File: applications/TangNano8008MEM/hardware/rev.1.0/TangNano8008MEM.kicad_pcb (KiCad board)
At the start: 2 copper layers, 99.1 x 99.1 mm, 43 parts, among them J1 Barrel_Jack_Switch, J2 VCC_FPGA, J3 CPU Vcc, J4 TangNano20K5VInterface, J5 Conn_01x20, J6 Conn_01x20, J7 UART, J8 Conn_01x30, J9 Conn_01x30, SW1 SW_SPDT, SW2 INIT, SW3 HALT, U1 DCJ11, Y1 18MHz

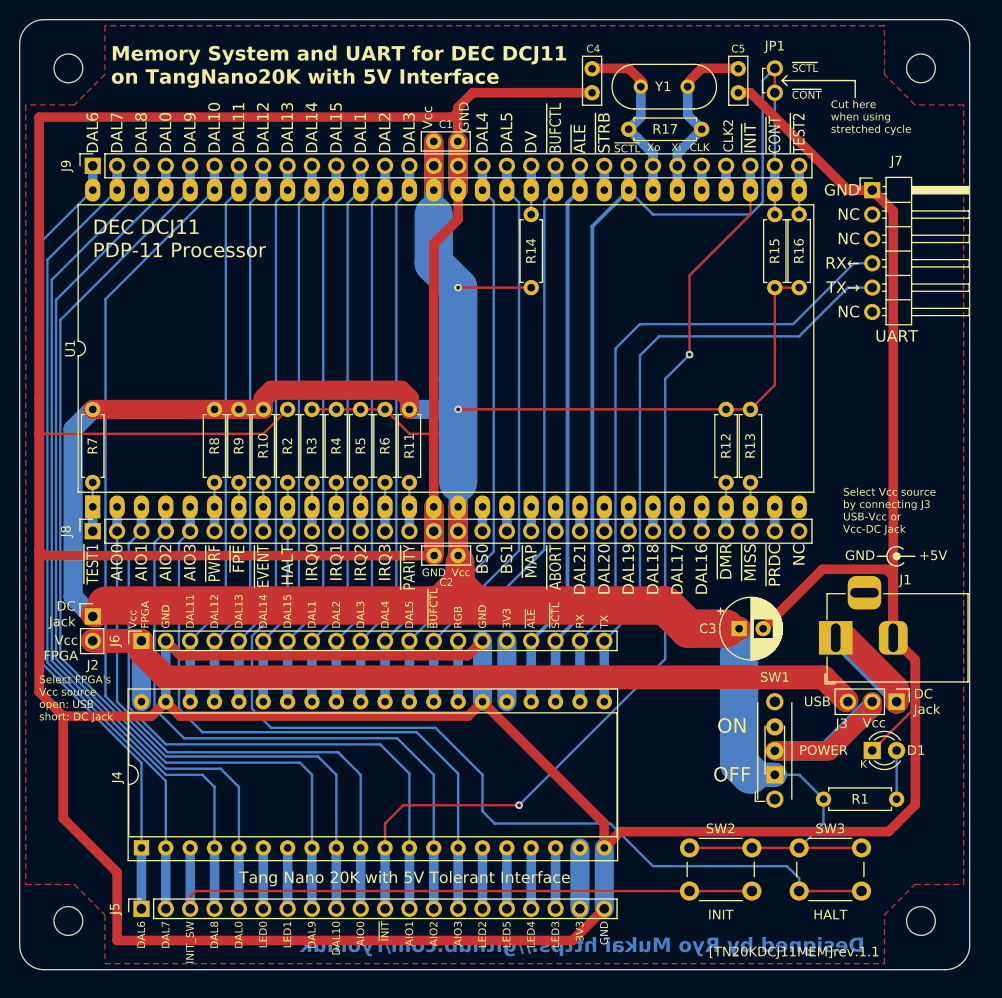
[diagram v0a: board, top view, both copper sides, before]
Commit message: PCB for 8008 updated
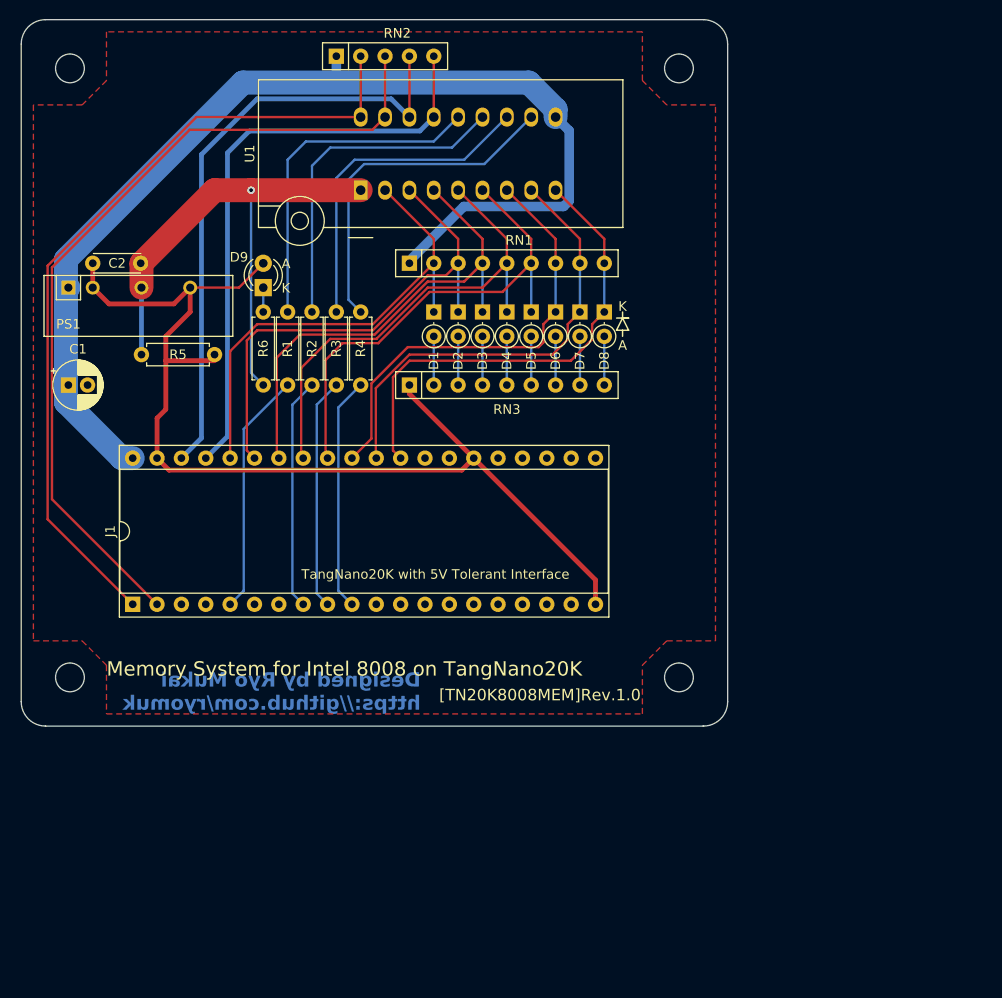
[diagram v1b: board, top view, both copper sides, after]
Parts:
- removed C3: 47uF, 000_MyFootprint:CP_Radial_D6.3mm_P2.50mm
- removed C4, C5: 68p, 000_MyFootprint:C_Disc_D5.0mm_W2.5mm_P2.50mm
- removed J2: VCC_FPGA, 000_MyFootprint:PinHeader_1x02_P2.54mm_Vertical
- removed J3: CPU Vcc, 000_MyFootprint:PinHeader_1x03_P2.54mm_Vertical
- removed J4: TangNano20K5VInterface, 000_MyFootprint:DIP-40_W15.24mm_Socket
- removed J5, J6: Conn_01x20, 000_MyFootprint:PinSocket_1x20_P2.54mm_Vertical
- removed J7: UART, 000_MyFootprint:PinHeader_1x06_P2.54mm_Horizontal
- removed J8, J9: Conn_01x30, 000_MyFootprint:PinSocket_1x30_P2.54mm_Vertical
- removed JP1: SCTL_CONT, 000_MyFootprint:JumperedPinHeader_1x02_P2.54mm_Vertical
- removed R10, R11, R12, R13, R14, R15, R16, R7, R8, R9: 100k, 000_MyFootprint:R_Axial_DIN0207_L6.3mm_D2.5mm_P7.62mm_Horizontal
- removed R17: 1M, 000_MyFootprint:R_Axial_DIN0207_L6.3mm_D2.5mm_P7.62mm_Horizontal
- removed the REF** at (94.0, 94.0)
- removed the REF** at (5.08, 5.08)
- removed the REF** at (91.4, 55.9)
- removed the REF** at (5.08, 94.0)
- removed the REF** at (94.0, 5.08)
- removed SW1: SW_SPDT, 000_MyFootprint:SW_SPDT_Toggle_with_mount
- removed SW2: INIT, 000_MyFootprint:SW_PUSH_6mm_H4.3mm
- removed SW3: HALT, 000_MyFootprint:SW_PUSH_6mm_H4.3mm
- removed Y1: 18MHz, 000_MyFootprint:Crystal_HC49-U_Vertical
- added D2: 1N4148, 000_MyFootprint:D_DO-35_SOD27_P2.54mm_Vertical_KathodeUp, F.Cu at (45.7, 30.5)
- added D3: 1N4148, 000_MyFootprint:D_DO-35_SOD27_P2.54mm_Vertical_KathodeUp, F.Cu at (48.3, 30.5)
- added D4: 1N4148, 000_MyFootprint:D_DO-35_SOD27_P2.54mm_Vertical_KathodeUp, F.Cu at (50.8, 30.5)
- added D5: 1N4148, 000_MyFootprint:D_DO-35_SOD27_P2.54mm_Vertical_KathodeUp, F.Cu at (53.3, 30.5)
- added D6: 1N4148, 000_MyFootprint:D_DO-35_SOD27_P2.54mm_Vertical_KathodeUp, F.Cu at (55.9, 30.5)
- added D7: 1N4148, 000_MyFootprint:D_DO-35_SOD27_P2.54mm_Vertical_KathodeUp, F.Cu at (58.4, 30.5)
- added D8: 1N4148, 000_MyFootprint:D_DO-35_SOD27_P2.54mm_Vertical_KathodeUp, F.Cu at (61.0, 30.5)
- added D9: LED, 000_MyFootprint:LED_D3.0mm, F.Cu at (25.4, 27.9)
- added PS1: MAU103, 000_MyFootprint:SIP-6_without_3_5pin_for_DCDC_MAU, F.Cu at (5.08, 27.9)
- added REF**: MountingHole_3mm, 000_MyFootprint:MountingHole_3mm, F.Cu at (68.7, 5.08)
- added REF**: MountingHole_3mm, 000_MyFootprint:MountingHole_3mm, F.Cu at (68.7, 68.6)
- added REF**: MountingHole_3mm, 000_MyFootprint:MountingHole_3mm, F.Cu at (5.24, 5.08)
- added REF**: MountingHole_3mm, 000_MyFootprint:MountingHole_3mm, F.Cu at (5.24, 68.6)
- added RN1: 4.7k, Resistor_THT:R_Array_SIP9, F.Cu at (40.6, 25.4)
- added RN2: 1k, Resistor_THT:R_Array_SIP5, F.Cu at (33.0, 3.81)
- added RN3: 4.7k, Resistor_THT:R_Array_SIP9, F.Cu at (40.6, 38.1)
- C1: value 0.33uF -> 2.2uF; footprint 000_MyFootprint:C_Disc_D5.0mm_W2.5mm_P2.50mm -> 000_MyFootprint:CP_Radial_D5.0mm_P2.00mm
- C2: value 0.33uF -> 1uF; footprint 000_MyFootprint:C_Disc_D5.0mm_W2.5mm_P2.50mm -> 000_MyFootprint:C_Disc_D4.7mm_W2.5mm_P5.00mm
- D1: value LED -> 1N4148; footprint 000_MyFootprint:LED_D3.0mm -> 000_MyFootprint:D_DO-35_SOD27_P2.54mm_Vertical_KathodeUp
- J1: value Barrel_Jack_Switch -> TangNano20K5VInterface; footprint 000_MyFootprint:BarrelJack_Horizontal -> 000_MyFootprint:DIP-40_W15.24mm_Socket
- R1, R2, R3, R4, R5: value 100k -> 1k
- U1: value DCJ11 -> intel8008; footprint 000_MyFootprint:DIP-60_W33.02mm_LongPads -> 000_MyFootprint:DIP_Socket-18_W4.3_W5.08_W7.62_W10.16_W10.9_3M_218-3341-00-0602J
- moved R1 81.3 mm to (27.9, 30.5), turned to -90 degrees
- moved J1 73.4 mm to (11.8, 61.0), turned to 90 degrees
- moved D1 64.7 mm to (43.2, 30.5), turned to -90 degrees
- moved C2 48.8 mm to (7.62, 25.4), turned to 0 degrees
- moved C1 45.8 mm to (5.08, 38.1)
- moved U1 43.3 mm to (35.6, 17.8)
- moved R5 16.3 mm to (20.3, 34.9), turned to 180 degrees
- moved R6 16.3 mm to (25.4, 30.5)
- moved R2 10.5 mm to (30.5, 30.5)
- moved R3 10.5 mm to (33.0, 30.5)
- moved R4 10.5 mm to (35.6, 30.5)
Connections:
- C1 pad 1: VCC -> +5V
- C2 pad 1: VCC -> GND
- C2 pad 2: GND -> -9V
- D1 pad 1: GND -> D7
- J1 pad 1: Net-(J3-Pin_1) -> INTERRUPT
- J1 pad 2: GND -> READY
- R1 pad 1: Net-(D1-A) -> Net-(U1-SYNC)
- R1 pad 2: VCC -> SYNC
- R2 pad 1: GND -> Net-(U1-S0)
- R2 pad 2: HALT -> S0
- R3 pad 1: GND -> Net-(U1-S1)
- R3 pad 2: IRQ0 -> S1
- R4 pad 1: GND -> Net-(U1-S2)
- R4 pad 2: IRQ1 -> S2
- R5 pad 2: IRQ2 -> -9V
- R6 pad 1: GND -> Net-(D9-K)
- R6 pad 2: IRQ3 -> -9V
- U1 pad 1: TEST1_n -> -9V
- U1 pad 10: IRQ0 -> +5V
- U1 pad 11: IRQ1 -> Net-(U1-S2)
- U1 pad 12: IRQ2 -> Net-(U1-S1)
- U1 pad 13: IRQ3 -> Net-(U1-S0)
- U1 pad 14: PARITY_n -> Net-(U1-SYNC)
- U1 pad 15: GND -> CLK2
- U1 pad 16: VCC -> CLK1
- U1 pad 17: BS0 -> READY
- U1 pad 18: BS1 -> INTERRUPT
- U1 pad 2: AIO0 -> D7
- U1 pad 3: AIO1 -> D6
- U1 pad 4: AIO2 -> D5
- U1 pad 5: AIO3 -> D4
- U1 pad 6: PWRF_n -> D3
- U1 pad 7: FPE_n -> D2
- U1 pad 8: EVENT_n -> D1
- U1 pad 9: HALT -> D0
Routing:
- net GND: track 614.9 -> 112.0 mm
- net VCC: track 323.7 -> 0.00 mm, vias 2 -> 0
- net +5V: track 0.00 -> 125.8 mm
- net CONT_n: track 104.3 -> 0.00 mm
- net DAL9: track 102.1 -> 0.00 mm
- net DAL10: track 101.5 -> 0.00 mm
- net INIT_n: track 100.3 -> 0.00 mm, vias 2 -> 0
- net HALT: track 99.6 -> 0.00 mm
- net DAL0: track 95.4 -> 0.00 mm
- net DAL8: track 90.6 -> 0.00 mm
- net VCC_FPGA: track 88.3 -> 0.00 mm
- net READY: track 0.00 -> 87.2 mm
- net DAL7: track 85.6 -> 0.00 mm
- net INTERRUPT: track 0.00 -> 84.4 mm
- net DAL6: track 83.9 -> 0.00 mm
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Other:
- board size 99.1 x 99.1 mm -> 73.7 x 73.7 mm
- board text added: "A"
- board text added: "Memory System for Intel 8008 on TangNano20K"
- board text added: "TangNano20K with 5V Tolerant Interface"
- board text added: "[TN20K8008MEM]Rev.1.0"
- board text removed: "3V3"
- board text removed: "AIO0"
- board text removed: "AIO1"
- board text removed: "AIO2"
- board text removed: "AIO3"
- board text removed: "BS0"
- board text removed: "BS1"
- board text removed: "CLK"
- board text removed: "CLK2"
- board text removed: "Cut here when using stretched cycle"
- board text removed: "DAL0"
- board text removed: "DAL1"
- board text removed: "DAL10"
- board text removed: "DAL11"
- board text removed: "DAL12"
- board text removed: "DAL13"
- board text removed: "DAL14"
- board text removed: "DAL15"
- board text removed: "DAL16"
- board text removed: "DAL17"
- board text removed: "DAL18"
- board text removed: "DAL19"
- board text removed: "DAL2"
- board text removed: "DAL20"
- board text removed: "DAL21"
- board text removed: "DAL3"
- board text removed: "DAL4"
- board text removed: "DAL5"
- board text removed: "DAL6"
- board text removed: "DAL7"
- board text removed: "DAL8"
- board text removed: "DAL9"
- board text removed: "DC Jack"
- board text removed: "DEC DCJ11 PDP-11 Processor"
- board text removed: "DV"
- board text removed: "GND"
- board text removed: "HALT"
- board text removed: "INIT_SW"
- board text removed: "IRQ0"
- board text removed: "IRQ1"
- board text removed: "IRQ2"
- board text removed: "IRQ3"
- board text removed: "LED0"
- board text removed: "LED1"
- board text removed: "LED2"
- board text removed: "LED3"
- board text removed: "LED4"
- board text removed: "LED5"
- board text removed: "Memory System and UART for DEC DCJ11 on TangNano20K with 5V Interface"
- board text removed: "NC"
- board text removed: "OFF"
- board text removed: "ON"
- board text removed: "POWER"
- board text removed: "RGB"
- board text removed: "RX"
- board text removed: "RX←"
- board text removed: "Select FPGA's Vcc source open: USB short: DC Jack"
- board text removed: "Select Vcc source by connecting J3 USB-Vcc or Vcc-DC Jack"
- board text removed: "TX"
- board text removed: "TX→"
- board text removed: "Tang Nano 20K with 5V Tolerant Interface"
- board text removed: "USB"
- board text removed: "Vcc"
- board text removed: "Vcc FPGA"
- board text removed: "Xi"
- board text removed: "Xo"
- board text removed: "[TN20KDCJ11MEM]rev.1.1"
- board text removed: "~{ABORT}"
- board text removed: "~{ALE}"
- board text removed: "~{BUFCTL}"
- board text removed: "~{CONT}"
- board text removed: "~{DMR}"
- board text removed: "~{EVENT}"
- board text removed: "~{FPE}"
- board text removed: "~{INIT}"
- board text removed: "~{MAP}"
- board text removed: "~{MISS}"
- board text removed: "~{PARITY}"
- board text removed: "~{PRDC}"
- board text removed: "~{PWRF}"
- board text removed: "~{SCTL}"
- board text removed: "~{STRB}"
- board text removed: "~{TEST1}"
- board text removed: "~{TEST2}"
